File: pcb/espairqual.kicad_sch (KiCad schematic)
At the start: 31 parts, among them J1 24VAC, J2 PMSX003, J3 USB_C_Receptacle_USB2.0, J7 eflashy32, U1 BD9G101G, U2 ESP32-WROOM-32D, U3 AMS1117-3.3

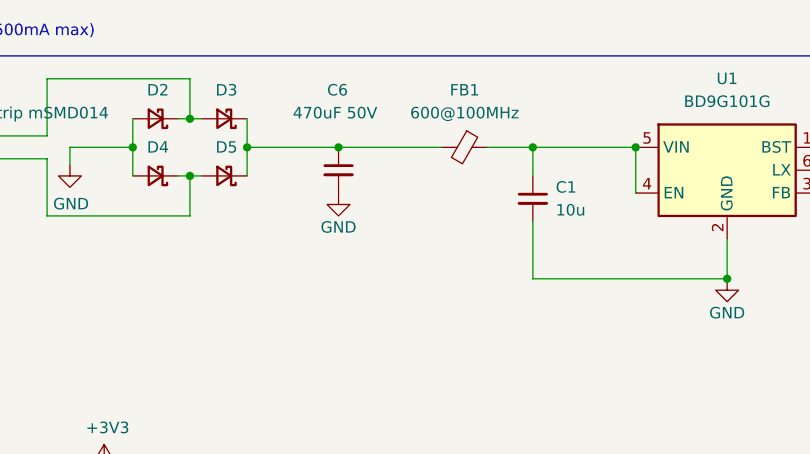
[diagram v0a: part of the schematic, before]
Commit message: caps
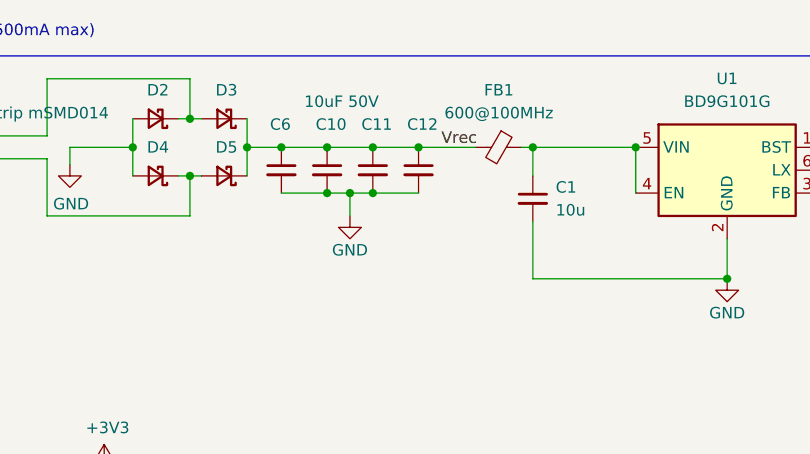
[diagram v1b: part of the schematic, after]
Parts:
- added C10, C11, C12: 10uF 50V, Capacitor_SMD:C_1206_3216Metric, symbol Device:C_Small
- C6: value 470uF 50V -> 10uF 50V; footprint Capacitor_SMD:CP_Elec_10x10 -> Capacitor_SMD:C_1206_3216Metric; LCSC C125977 -> C13585
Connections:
- net GND: now also C10.2, C11.2, C12.2
- net Vrec: now reaches C6.1, D3.1 (K), D5.1 (K), FB1.2
- net Vrec: now also C10.1, C11.1, C12.1
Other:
- moved on the sheet: FB1
